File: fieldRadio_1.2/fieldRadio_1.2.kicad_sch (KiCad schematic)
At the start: 11 parts, among them J1 Conn_01x02, J12 AudioJack3_Switch, J18 Conn_01x16, J2 Conn_01x02, J3 Conn_01x03, J4 AudioJack2_Switch, J5 AudioJack3_Switch, J7 Conn_01x04, J8 Conn_01x12

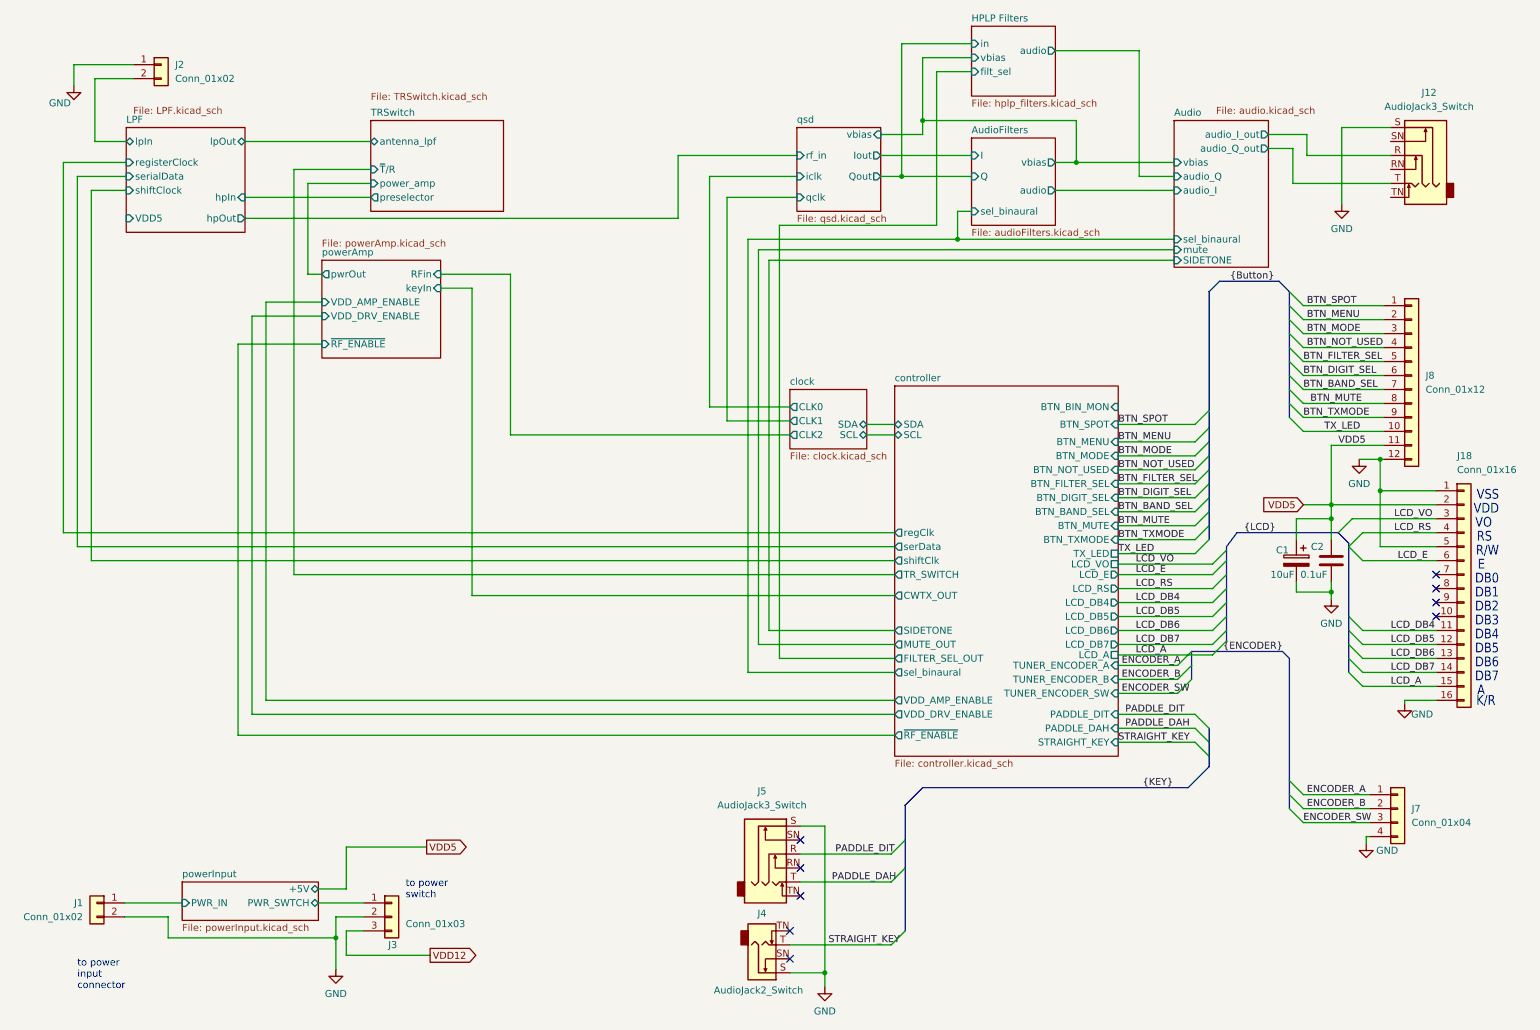
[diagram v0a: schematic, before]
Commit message: Working on fieldRadio_1.2 schematics
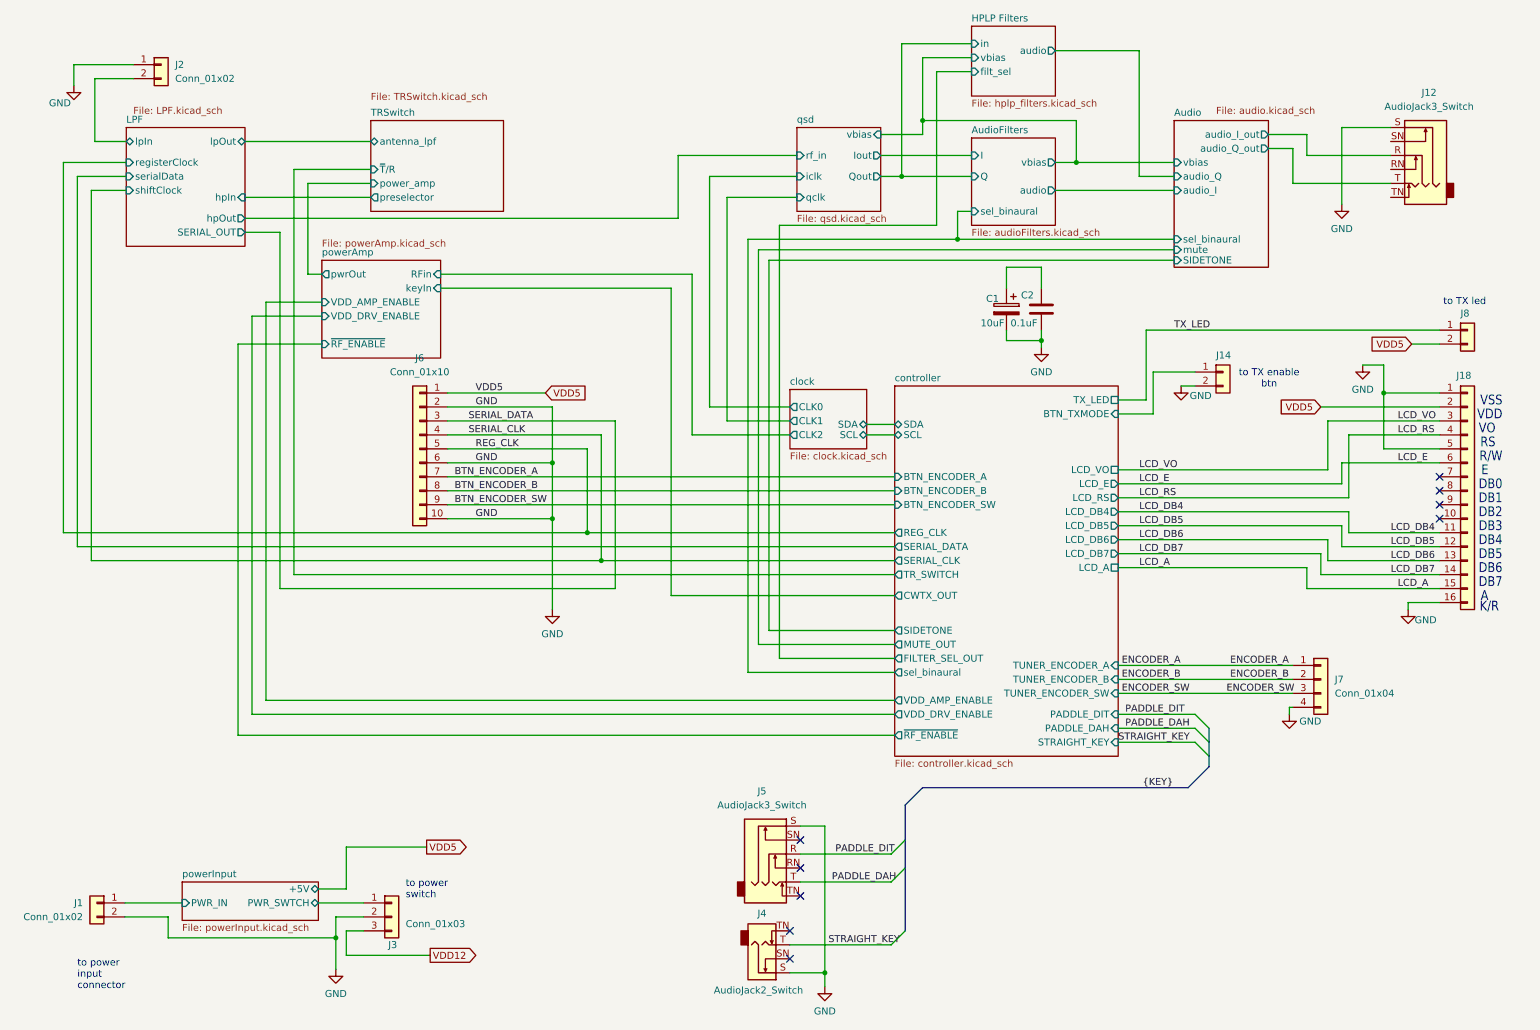
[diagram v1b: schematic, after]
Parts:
- removed J8: Conn_01x12, Connector_PinHeader_2.54mm:PinHeader_1x12_P2.54mm_Vertical, symbol Connector_Generic:Conn_01x12
- added J14, J8: Conn_01x02, Connector_PinHeader_2.54mm:PinHeader_1x02_P2.54mm_Vertical, symbol Connector_Generic:Conn_01x02
- added J6: Conn_01x10, symbol Connector_Generic:Conn_01x10
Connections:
- net GND: now also J14.2 (Pin_2), J6.10 (Pin_10), J6.2 (Pin_2), J6.6 (Pin_6)
- net TX_LED: now also J8.1 (Pin_1)
- net VDD5: now also J6.1 (Pin_1), J8.2 (Pin_2); no longer C1.1, C2.1
- new net: C1.1, C2.1
- new net BTN_ENCODER_A: J6.7 (Pin_7)
- new net BTN_ENCODER_B: J6.8 (Pin_8)
- new net BTN_ENCODER_SW: J6.9 (Pin_9)
- new net REG_CLK: J6.5 (Pin_5)
- new net SERIAL_CLK: J6.4 (Pin_4)
- new net SERIAL_DATA: J6.3 (Pin_3)
- new net controller/BTN_TXMODE: J14.1 (Pin_1)
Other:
- sheet LPF ports: added SERIAL_OUT; removed VDD5
- sheet controller ports: added BTN_ENCODER_A, BTN_ENCODER_B, BTN_ENCODER_SW, REG_CLK, SERIAL_CLK, SERIAL_DATA; removed BTN_BAND_SEL, BTN_BIN_MON, BTN_DIGIT_SEL, BTN_FILTER_SEL, BTN_MENU, BTN_MODE, BTN_MUTE, BTN_NOT_USED, BTN_SPOT, regClk, serData, shiftClk
- note added: "to TX enable btn"
- note added: "to TX led"
- moved on the sheet: C1, C2, J18, J7
